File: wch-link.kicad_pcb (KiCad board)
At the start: 2 copper layers, 37 x 16 mm, 35 parts, among them J1 USB2.0_C_v3, M1 M2-Hole, M2 M2-Hole, M3 M2-Hole, M4 M2-Hole, U1 AMS1117-3.3, U2 CH32V305FBP6, Y1 Oscillator_24GND

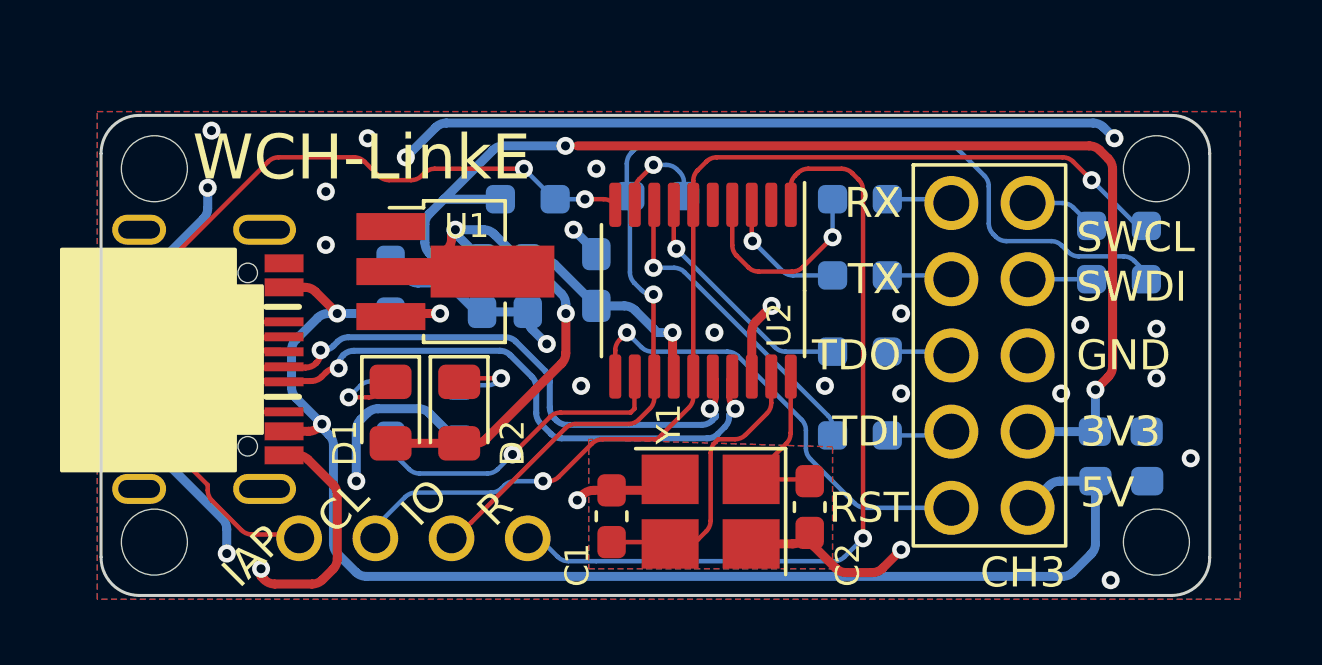
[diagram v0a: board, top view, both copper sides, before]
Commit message: v1.1.0
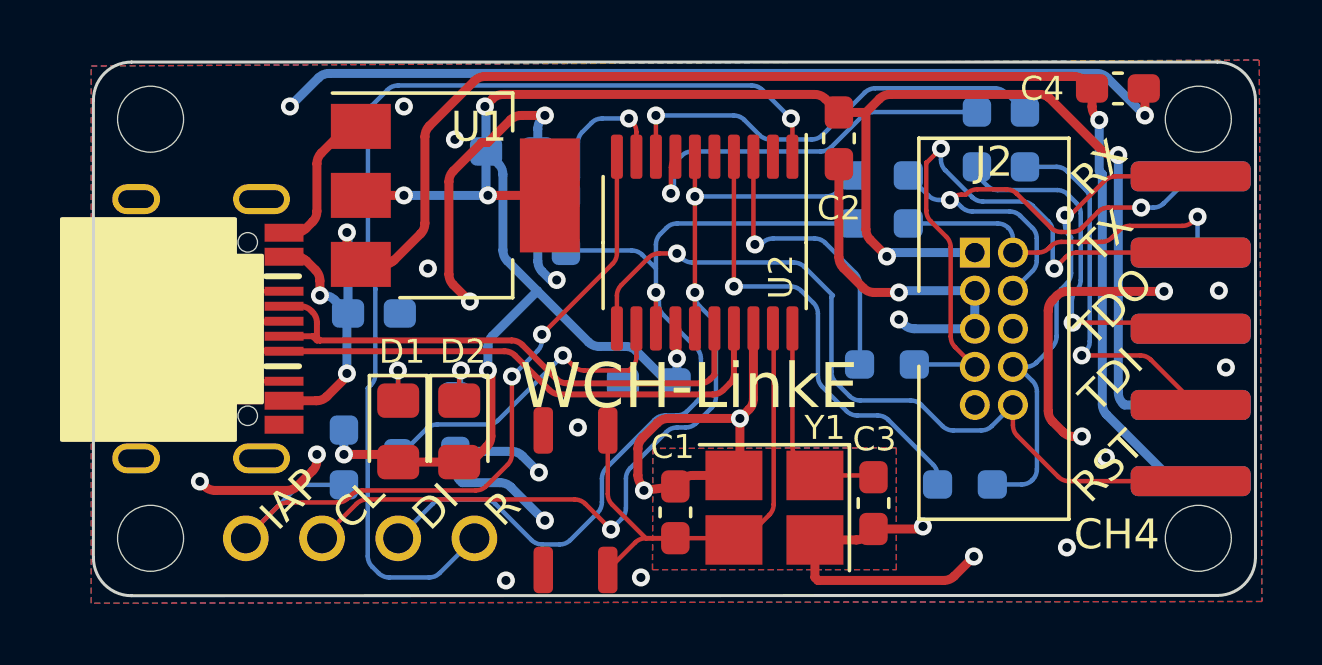
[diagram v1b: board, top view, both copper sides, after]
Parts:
- removed the C6 at (71.6, 40.4)
- added J2: SWD-Debugger_Side-10Pin, $74th:BoxPinHeader_2x05_P1.27mm_Vertical, F.Cu at (87.2, 41.9)
- added SW1: SW_Push, $74th:SKRPABE010, F.Cu at (73.2, 47.6)
- C2: renamed from C3; moved to F.Cu
- C4: moved to F.Cu
- CH1: renamed from CH4; value RT -> IAP
- CH4: renamed from CH3; footprint $74th:WCH-Link-Port -> $74th:Side-2x5P-PinHeader-Right
- U1: footprint $74th:Regulator_AMS1117_SOT-89 -> Package_TO_SOT_SMD:SOT-223-3_TabPin2
- Y1: value Oscillator_24GND -> 12M
- moved C2 13.6 mm to (82.0, 35.7), turned to 90 degrees
- moved C4 13.1 mm to (91.4, 33.9)
- moved R1 11.3 mm to (88.2, 35.6), turned to -90 degrees
- moved R10 10.6 mm to (65.5, 46.2), turned to -90 degrees
- moved R3 10.1 mm to (86.2, 47.1), turned to 0 degrees
- moved REF** 9.42 mm to (76.2, 34.3)
- moved R6 8.15 mm to (83.4, 38.4), turned to 0 degrees
- moved R5 8.11 mm to (83.4, 36.8), turned to 0 degrees
- moved R2 8.08 mm to (86.6, 35.6), turned to -90 degrees
- moved CH4 6.77 mm to (93.7, 41.9)
- moved C6 4.48 mm to (71.0, 36.0), turned to 0 degrees
- moved C5 3.80 mm to (75.8, 43.7), turned to 180 degrees
- moved R7 3.18 mm to (72.9, 38.4), turned to -90 degrees
- moved R4 3.10 mm to (83.6, 43.1), turned to 0 degrees
- moved U1 2.54 mm to (69.2, 37.5)
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- renumbered C2 to C3, C7 to C6, C8 to C7, CH1 to CH2, CH2 to CH3, R6 to R1, R8 to R10, R5 to R2, R1 to R5, R2 to R6, R9 to R8, R10 to R9
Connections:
- net D_SWCLK renamed /D_SWCLK
- net D_SWDIO renamed /D_SWDIO
- net Net-(U2-OSC_IN/PD0) renamed /ModeS
- net RT renamed /RT
- net USB_N renamed /USBD-
- net USB_P renamed /USBD+
- CH4 pad 1: Net-(CH3-RX) -> /RX
- CH4 pad 10: Net-(CH3-SWCLK) -> +5V
- CH4 pad 2: Net-(CH3-TX) -> /SWCLK/TCK
- CH4 pad 3: Net-(CH3-TDO) -> /TX
- CH4 pad 4: Net-(CH3-TDI) -> /SWDIO/TMS
- CH4 pad 5: RST -> /TDO
- CH4 pad 6: +5V -> GND
- CH4 pad 7: +3V3 -> /TDI
- CH4 pad 8: GND -> +3V3
- CH4 pad 9: Net-(CH3-SWDIO) -> RST
- R1 pad 1: Net-(CH3-TDI) -> Net-(U2-PB15)
- R1 pad 2: TDI -> /TDI
- R2 pad 1: Net-(CH3-TDO) -> Net-(U2-PB14)
- R2 pad 2: TDO -> /TDO
- R3 pad 1: Net-(CH3-RX) -> Net-(U2-PB11)
- R3 pad 2: RX -> /RX
- R4 pad 1: Net-(CH3-TX) -> Net-(U2-PB10)
- R4 pad 2: TX -> /TX
- R5 pad 2: Net-(CH3-SWCLK) -> /SWCLK/TCK
- R6 pad 2: Net-(CH3-SWDIO) -> /SWDIO/TMS
- U2 pad 3: TX -> Net-(U2-PB10)
- U2 pad 4: RX -> Net-(U2-PB11)
- U2 pad 7: TDO -> Net-(U2-PB14)
- U2 pad 8: TDI -> Net-(U2-PB15)
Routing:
- net GND: track 69.2 -> 107.4 mm, vias 30 -> 27
- net /TX: track 0.00 -> 21.4 mm, vias 0 -> 2
- net /SWCLK/TCK: track 0.00 -> 16.6 mm, vias 0 -> 2
- net /RX: track 0.00 -> 16.5 mm, vias 0 -> 1
- net Net-(U2-PB11): track 0.00 -> 15.5 mm, vias 0 -> 1
- net Net-(U2-PB15): track 0.00 -> 14.9 mm, vias 0 -> 1
- net Net-(U2-PB14): track 0.00 -> 13.0 mm, vias 0 -> 1
- net /SWDIO/TMS: track 0.00 -> 12.5 mm, vias 0 -> 1
- net /TDI: track 0.00 -> 12.4 mm, vias 0 -> 1
- net /TDO: track 0.00 -> 12.0 mm, vias 0 -> 1
- net RST: track 15.3 -> 26.7 mm
- net TDI: track 10.6 -> 0.00 mm, vias 1 -> 0
- net +3V3: track 65.0 -> 75.1 mm, vias 5 -> 8
- net Net-(U2-PB10): track 0.00 -> 9.90 mm, vias 0 -> 1
- net /RT: track 27.2 -> 35.6 mm
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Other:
- board size 37 x 16 mm -> 38.7 x 17.8 mm
- board text added: "3V3"
- board text added: "5V"
- board text added: "DI"
- board text added: "GND"
- board text added: "RST"
- board text added: "RX"
- board text added: "SWCLK"
- board text added: "SWDIO"
- board text added: "TCK"
- board text added: "TDI"
- board text added: "TDO"
- board text added: "TMS"
- board text added: "TX"
- board text added: "v1.1.0"
- board text removed: "IO"
- board text removed: "v1.0.0"
